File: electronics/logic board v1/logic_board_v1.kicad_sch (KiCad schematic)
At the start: 48 parts, among them J1 Screw_Terminal_01x02, J2 SWD, J3 Conn_01x04, J4 USB_B_Micro, Q1 AO3401A, SW1 SW_SPDT, U1 STM32F405RGTx, U3 USBLC6-2SC6, Y1 16MHz

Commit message: Update logic_board_v1.kicad_sch
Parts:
- C13, C15, C16, C17: footprint (none) -> Capacitor_SMD:C_0603_1608Metric
- C14, C18: footprint (none) -> Capacitor_SMD:C_0402_1005Metric
- D1, D3: footprint (none) -> LED_SMD:LED_0603_1608Metric
- D2: footprint (none) -> Diode_SMD:D_0201_0603Metric
- R1, R10, R11, R13, R3, R4, R5, R8, R9: footprint (none) -> Resistor_SMD:R_0603_1608Metric
- R12, R2, R6, R7: footprint (none) -> Resistor_SMD:R_0402_1005Metric
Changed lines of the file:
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@@
 			)
 		)
-		(property "Footprint" ""
+		(property "Footprint" "Resistor_SMD:R_0603_1608Metric"
 			(at 110.49 147.32 0)
 			(effects
@@
 			)
 		)
-		(property "Footprint" ""
+		(property "Footprint" "Resistor_SMD:R_0603_1608Metric"
 			(at 92.71 173.99 0)
 			(effects
@@
 			)
 		)
-		(property "Footprint" ""
+		(property "Footprint" "Resistor_SMD:R_0603_1608Metric"
 			(at 97.79 146.05 0)
 			(effects
@@
 			)
 		)
-		(property "Footprint" ""
+		(property "Footprint" "Resistor_SMD:R_0603_1608Metric"
 			(at 95.25 146.05 0)
 			(effects
@@
 			)
 		)
-		(property "Footprint" ""
+		(property "Footprint" "Resistor_SMD:R_0603_1608Metric"
 			(at 170.18 38.1 0)
 			(effects
@@
 			)
 		)
-		(property "Footprint" ""
+		(property "Footprint" "Diode_SMD:D_0201_0603Metric"
 			(at 46.99 21.59 90)
 			(effects
@@
 			)
 		)
-		(property "Footprint" ""
+		(property "Footprint" "Capacitor_SMD:C_0603_1608Metric"
 			(at 68.58 30.48 0)
 			(effects
@@
 			)
 		)
-		(property "Footprint" ""
+		(property "Footprint" "LED_SMD:LED_0603_1608Metric"
 			(at 232.41 30.48 90)
 			(effects
@@
 			)
 		)
-		(property "Footprint" ""
+		(property "Footprint" "Resistor_SMD:R_0603_1608Metric"
 			(at 92.71 30.48 0)
 			(effects
@@
 			)
 		)
-		(property "Footprint" ""
+		(property "Footprint" "Resistor_SMD:R_0402_1005Metric"
 			(at 149.86 34.29 0)
 			(effects
@@
 			)
 		)
-		(property "Footprint" ""
+		(property "Footprint" "Capacitor_SMD:C_0603_1608Metric"
 			(at 153.67 22.86 0)
 			(effects
@@
 			)
 		)
-		(property "Footprint" ""
+		(property "Footprint" "Resistor_SMD:R_0603_1608Metric"
 			(at 92.71 22.86 0)
 			(effects
@@
 			)
 		)
-		(property "Footprint" ""
+		(property "Footprint" "Capacitor_SMD:C_0603_1608Metric"
 			(at 63.5 30.48 0)
 			(effects
@@
 			)
 		)
-		(property "Footprint" ""
+		(property "Footprint" "Resistor_SMD:R_0402_1005Metric"
 			(at 149.86 19.05 0)
 			(effects
@@
 			)
 		)
-		(property "Footprint" ""
+		(property "Footprint" "Resistor_SMD:R_0402_1005Metric"
 			(at 106.68 104.14 0)
 			(effects
@@
 			)
 		)
-		(property "Footprint" ""
+		(property "Footprint" "Capacitor_SMD:C_0603_1608Metric"
 			(at 163.83 30.48 0)
 			(effects
@@
 			)
 		)
-		(property "Footprint" ""
+		(property "Footprint" "Capacitor_SMD:C_0402_1005Metric"
 			(at 77.47 30.48 0)
 			(effects
@@
 			)
 		)
-		(property "Footprint" ""
+		(property "Footprint" "LED_SMD:LED_0603_1608Metric"
 			(at 110.49 140.97 90)
 			(effects
@@
 			)
 		)
-		(property "Footprint" ""
+		(property "Footprint" "Resistor_SMD:R_0603_1608Metric"
 			(at 170.18 30.48 0)
 			(effects
@@
 			)
 		)
-		(property "Footprint" ""
+		(property "Footprint" "Resistor_SMD:R_0402_1005Metric"
 			(at 224.79 64.77 0)
 			(effects
@@
 			)
 		)
-		(property "Footprint" ""
+		(property "Footprint" "Resistor_SMD:R_0603_1608Metric"
 			(at 232.41 35.56 0)
 			(effects
@@
 			)
 		)
-		(property "Footprint" ""
+		(property "Footprint" "Capacitor_SMD:C_0402_1005Metric"
 			(at 118.11 26.67 0)
 			(effects

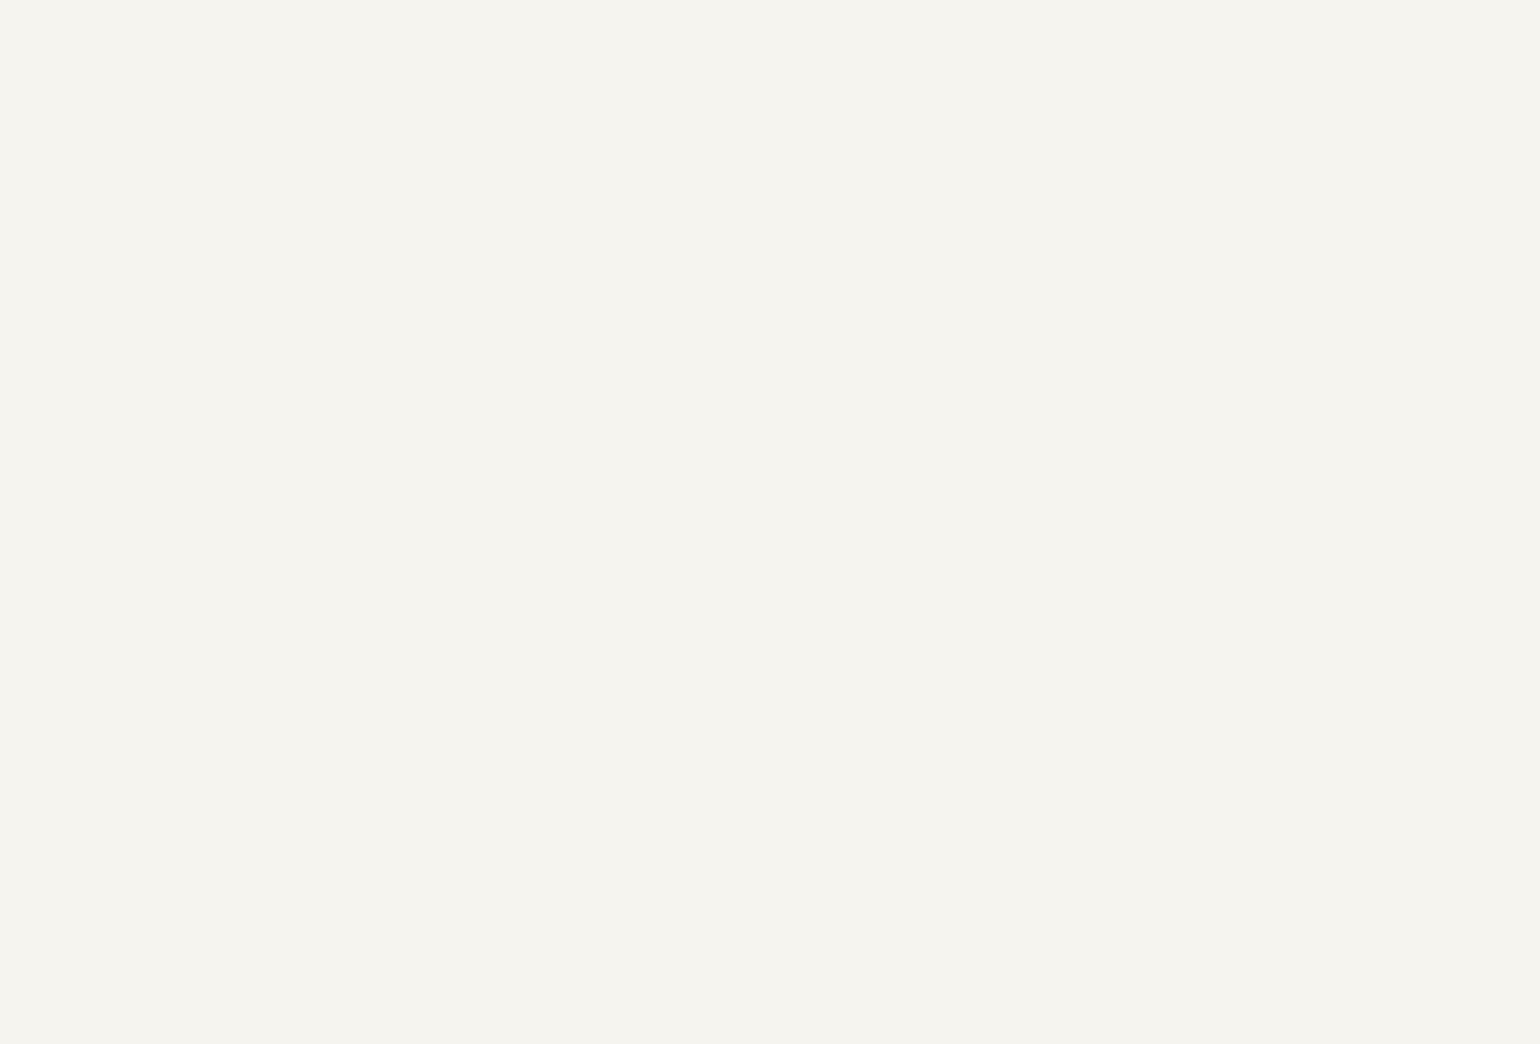
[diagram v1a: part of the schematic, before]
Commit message: Update logic_board_v1.kicad_sch
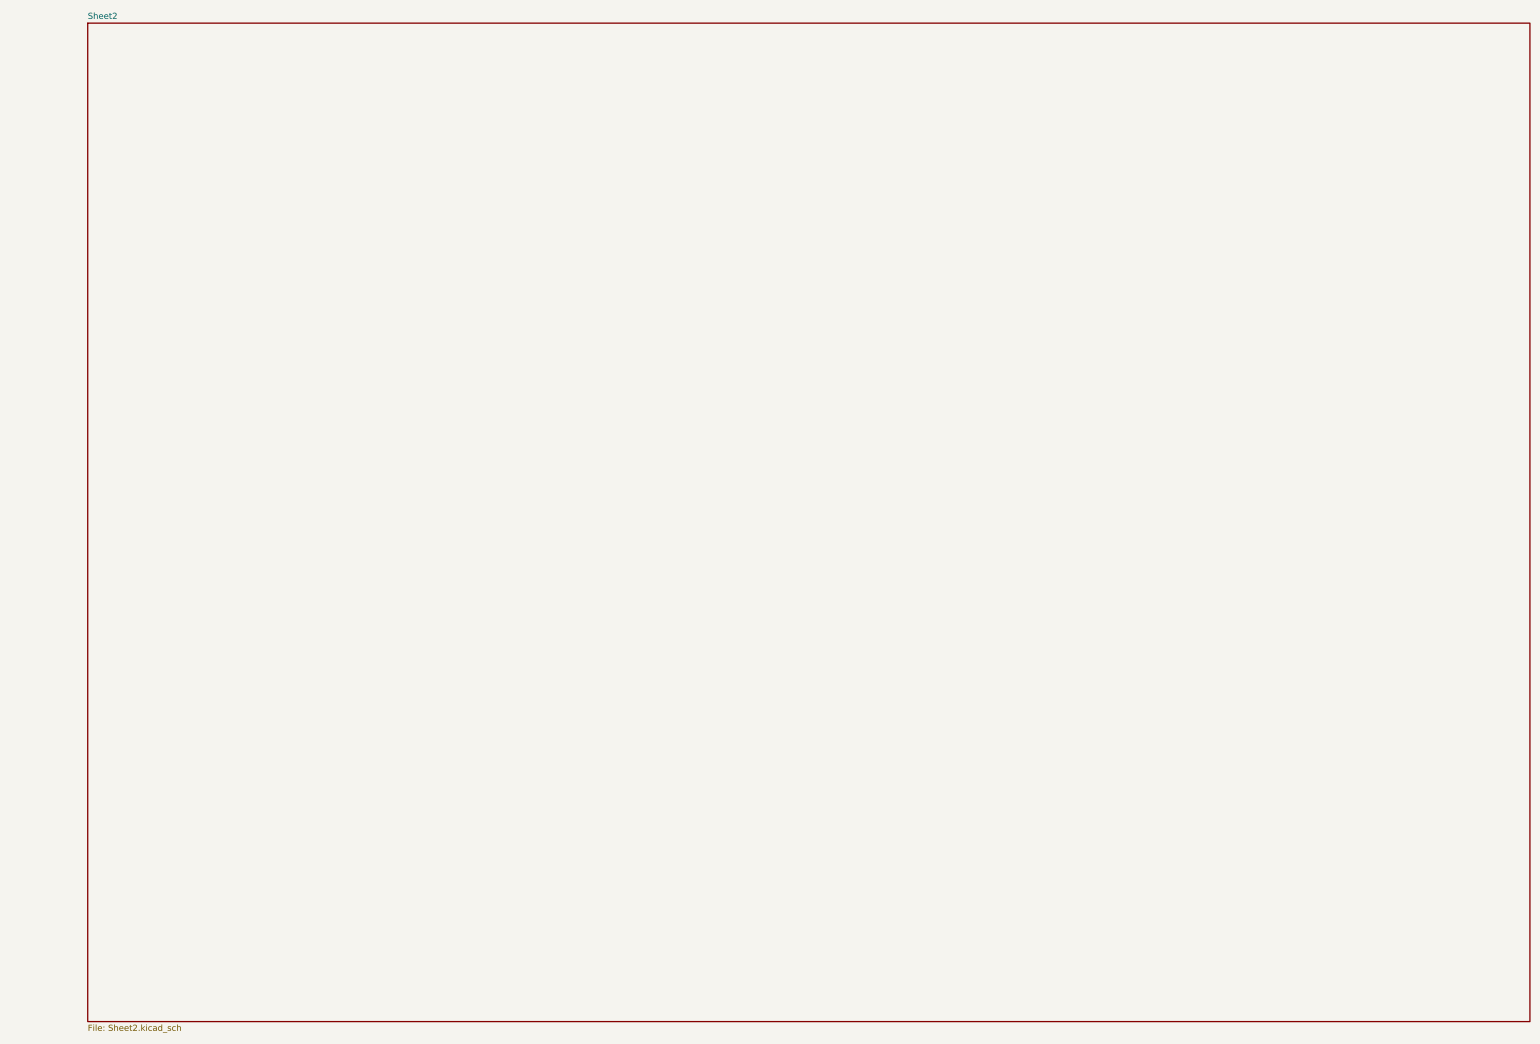
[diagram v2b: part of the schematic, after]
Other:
- added sheet Sheet2 (Sheet2.kicad_sch)
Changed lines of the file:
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@@
+		)
+	)
+	(sheet
+		(at 314.96 5.08)
+		(size 297.18 205.74)
+		(exclude_from_sim no)
+		(in_bom yes)
+		(on_board yes)
+		(dnp no)
+		(fields_autoplaced yes)
+		(stroke
+			(width 0.1524)
+			(type solid)
+		)
+		(fill
+			(color 0 0 0 0.0000)
+		)
+		(property "Sheetname" "Sheet2"
+			(at 314.96 4.3684 0)
+			(effects
+				(font
+					(size 1.27 1.27)
+				)
+				(justify left bottom)
+			)
+		)
+		(property "Sheetfile" "Sheet2.kicad_sch"
+			(at 314.96 211.4046 0)
+			(effects
+				(font
+					(size 1.27 1.27)
+				)
+				(justify left top)
+			)
+		)
+		(instances
+			(project "logic_board_v1"
+				(path "/3d6d34b6-2270-42d8-9a55-b901109db90f"
+					(page "2")
+				)
+			)
 		)
 	)
